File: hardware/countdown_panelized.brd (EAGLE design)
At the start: 38 x 40 mm, 30 parts, among them J1 BURNIN, J2 USB, J3 LiPo, J4 OLED, J5 TOP, J6 BASE, U1 DS3231MZ+TRL_SOIC8, U2 ATMEGA328P-AUR, U3 MCP73831T, U4 BL1551

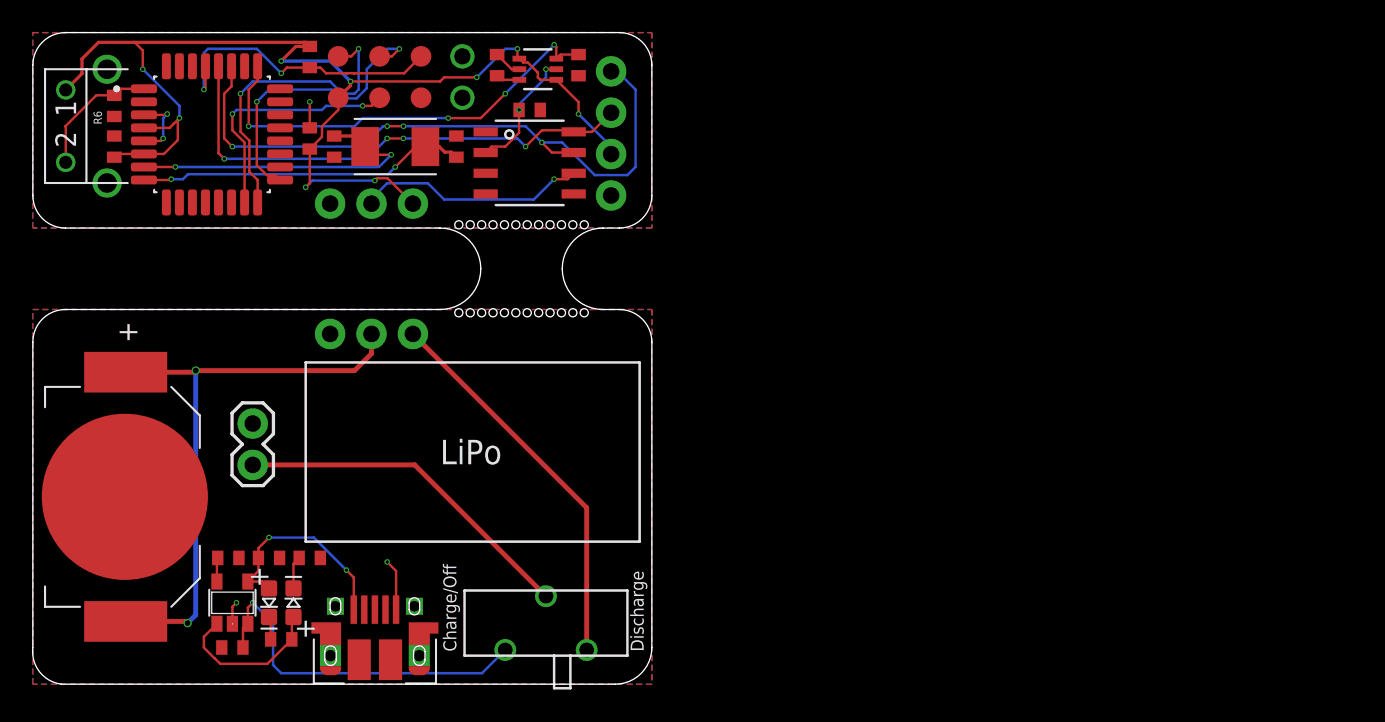
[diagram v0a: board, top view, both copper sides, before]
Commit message: prepare for order
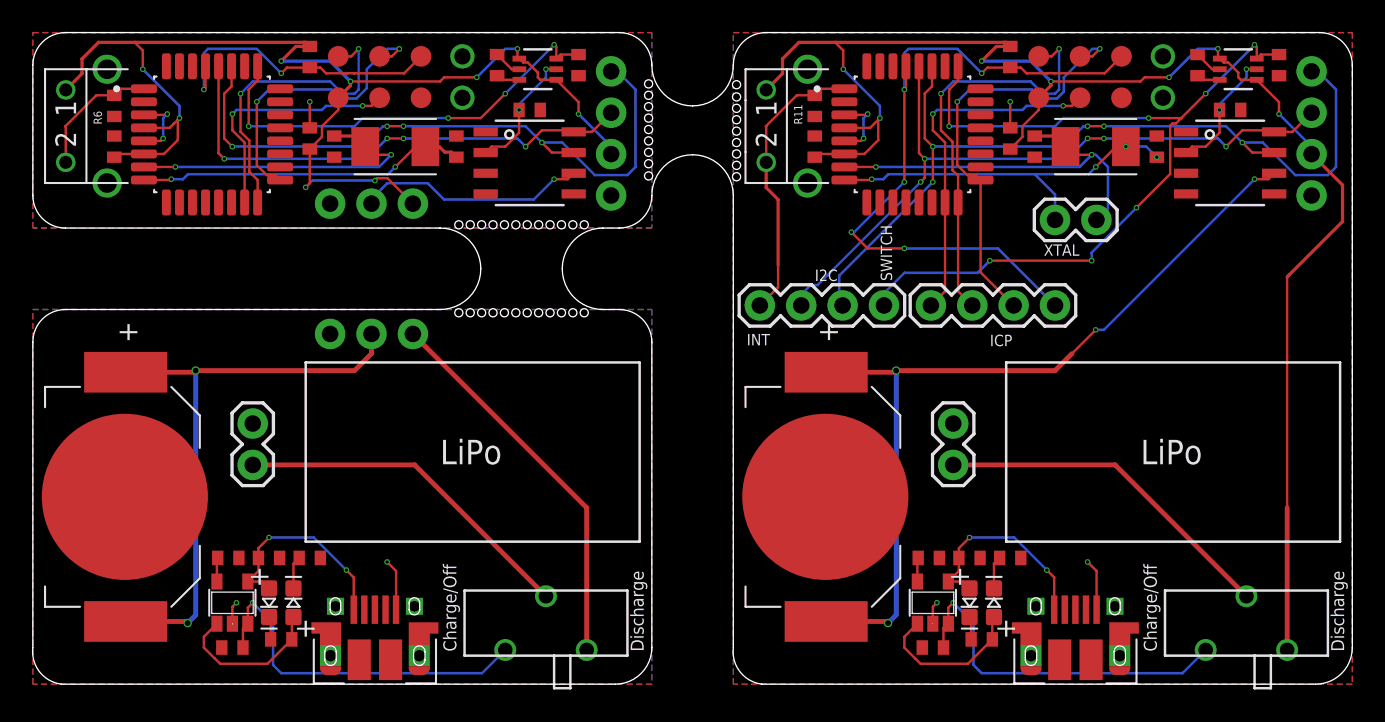
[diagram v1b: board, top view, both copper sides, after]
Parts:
- added BT2: BK-916-TR, scono:BAT_BK-916-TR
- added C10, C11: 0.1uF, scono:0402-CAP
- added C12: 1uF, scono:0402-CAP
- added C13, C14: 4.7uF, scono:0402-CAP
- added C8, C9: 20pF, scono:0402-CAP
- added D3, D4: (no value), scono:LED-0603
- added J10, J11: (no value), scono:1X04
- added J12: USB, scono:FCI_10103594-0001LF
- added J13: LiPo, scono:1X02
- added J7: BURNIN, scono:BURNIN
- added J8: OLED, scono:1X04_NO_SILK
- added J9: (no value), scono:1X02
- added R10, R11, R9: 10k, scono:R0402
- added R12, R14: 330R, scono:R0402
- added R13: 51k, scono:R0402
- added R8: 1k, scono:R0402
- added SW_INT1: FSMRACD, scono:FSMRACD
- added U$2: CL-SB-12C-12, scono:12C-12
- added U5: DS3231MZ+TRL_SOIC8, scono:SOIC-8
- added U6: ATMEGA328P-AUR, scono:QFP80P900X900X120-32N
- added U7: BL1551, scono:SOT-363
- added U8: MCP73831T, scono:SOT-23-5
- added Y2: (no value), scono:XTAL500X320X130N
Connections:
- new net AREF1: U6.20
- new net AVCC1: U6.18
- new net BAT+1: J13.2, U$2.2
- new net EN_CLK1: J10.1, R9.1, U6.25, U7.6
- new net GND: BT2.3, C10.1, C11.1, C12.1, C13.1, C14.1, C8.1, C9.1, J12.5, J13.1, J7.GND, J8.1, R10.2, R11.1, R13.1, R14.1, R9.2, U5.5, U6.21, U6.3, U6.5, U7.2, U8.2
- new net INT_WAKE1: J10.4, R11.2, SW_INT1.P$2, U6.1
- new net MISO1: J11.3, J7.MISO, U6.16
- new net MOSI1: J11.4, J7.MOSI, U6.15
- new net N$3: R10.1, U7.3
- new net N$5: D3.C, R12.2
- new net N$6: D4.C, R14.2
- new net PROG1: R13.2, U8.5
- new net RST1: J11.1, J7.RST, R8.2, U6.29
- new net SCK1: J11.2, J7.SCK, U6.17
- new net SCL1: J10.3, J8.3, U5.8, U6.28
- new net SDA1: J10.2, J8.4, U5.7, U6.27
- new net STAT1: D4.A, R12.1, U8.1
- new net VBAT_CHARGE1: C13.2, U$2.3, U8.3
- new net VCC: C10.2, C11.2, J7.3.3V, J8.2, R8.1, SW_INT1.P$1, U$2.1, U6.4, U6.6, U7.1, U7.4
- new net VCC_CLK1: C12.2, U5.2, U7.5
- new net VUSB1: C14.2, D3.A, J12.1, U8.4
- new net V_BAT: BT2.1, BT2.2, U5.6
- new net XTAL3: C9.2, J9.1, U6.8, Y2.1
- new net XTAL4: C8.2, J9.2, U6.7, Y2.2
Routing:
- net VCC: track 0.00 -> 96.2 mm, vias 0 -> 7
- net SDA1: track 0.00 -> 53.2 mm, vias 0 -> 5
- net EN_CLK1: track 0.00 -> 52.6 mm, vias 0 -> 7
- net V_BAT: track 0.00 -> 52.1 mm, vias 0 -> 4
- net SCL1: track 0.00 -> 43.6 mm, vias 0 -> 5
- net RST1: track 0.00 -> 43.1 mm, vias 0 -> 5
- net SCK1: track 0.00 -> 26.7 mm, vias 0 -> 2
- net MISO1: track 0.00 -> 25.7 mm, vias 0 -> 2
- net XTAL4: track 0.00 -> 24.3 mm, vias 0 -> 2
- net XTAL3: track 0.00 -> 23.6 mm, vias 0 -> 4
- net VBAT_CHARGE1: track 0.00 -> 22.4 mm, vias 0 -> 1
- net MOSI1: track 0.00 -> 21.9 mm, vias 0 -> 2
- net BAT+1: track 0.00 -> 21.3 mm
- net INT_WAKE1: track 0.00 -> 17.5 mm
- net VUSB1: track 0.00 -> 12.9 mm, vias 0 -> 2
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- added copper zone on layer 1, net GND
- added copper zone on layer 16, net GND
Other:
- board size 38 x 40 mm -> 81 x 40 mm
- board text added: "I2C"
- board text added: "ICP"
- board text added: "INT"
- board text added: "SWITCH"
- board text added: "XTAL"
